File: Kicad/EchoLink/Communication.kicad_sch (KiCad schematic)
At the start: 26 parts, among them J1 142-0701-801, J2 Conn_01x03_Pin, U2 E22-400M33S, U3 HM11, U4 MAX3221IPWR

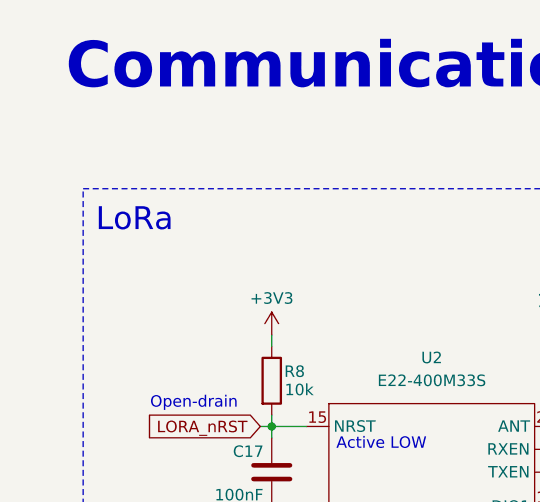
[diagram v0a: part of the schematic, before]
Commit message: wip: connector and bms IOs
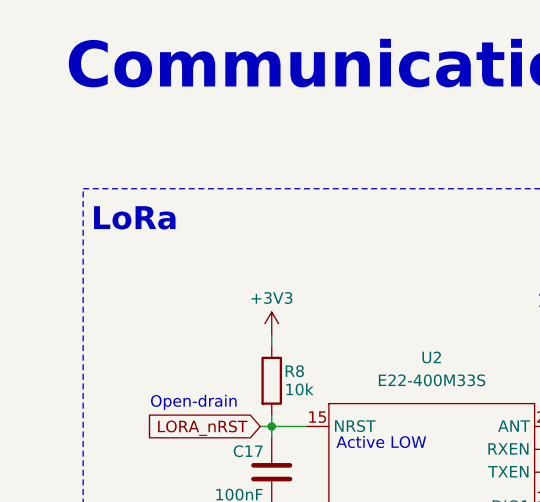
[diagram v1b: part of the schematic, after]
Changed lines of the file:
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@@
 			(font
 				(size 2.54 2.54)
-				(thickness 0.1875)
+				(thickness 0.508)
+				(bold yes)
 			)
 		)
